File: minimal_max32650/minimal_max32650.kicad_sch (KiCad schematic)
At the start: 38 parts, among them J1 FTSH-105-01-L-DV-K, U1 MAX32650GCE+, U2 ADP225ACPZ-R7

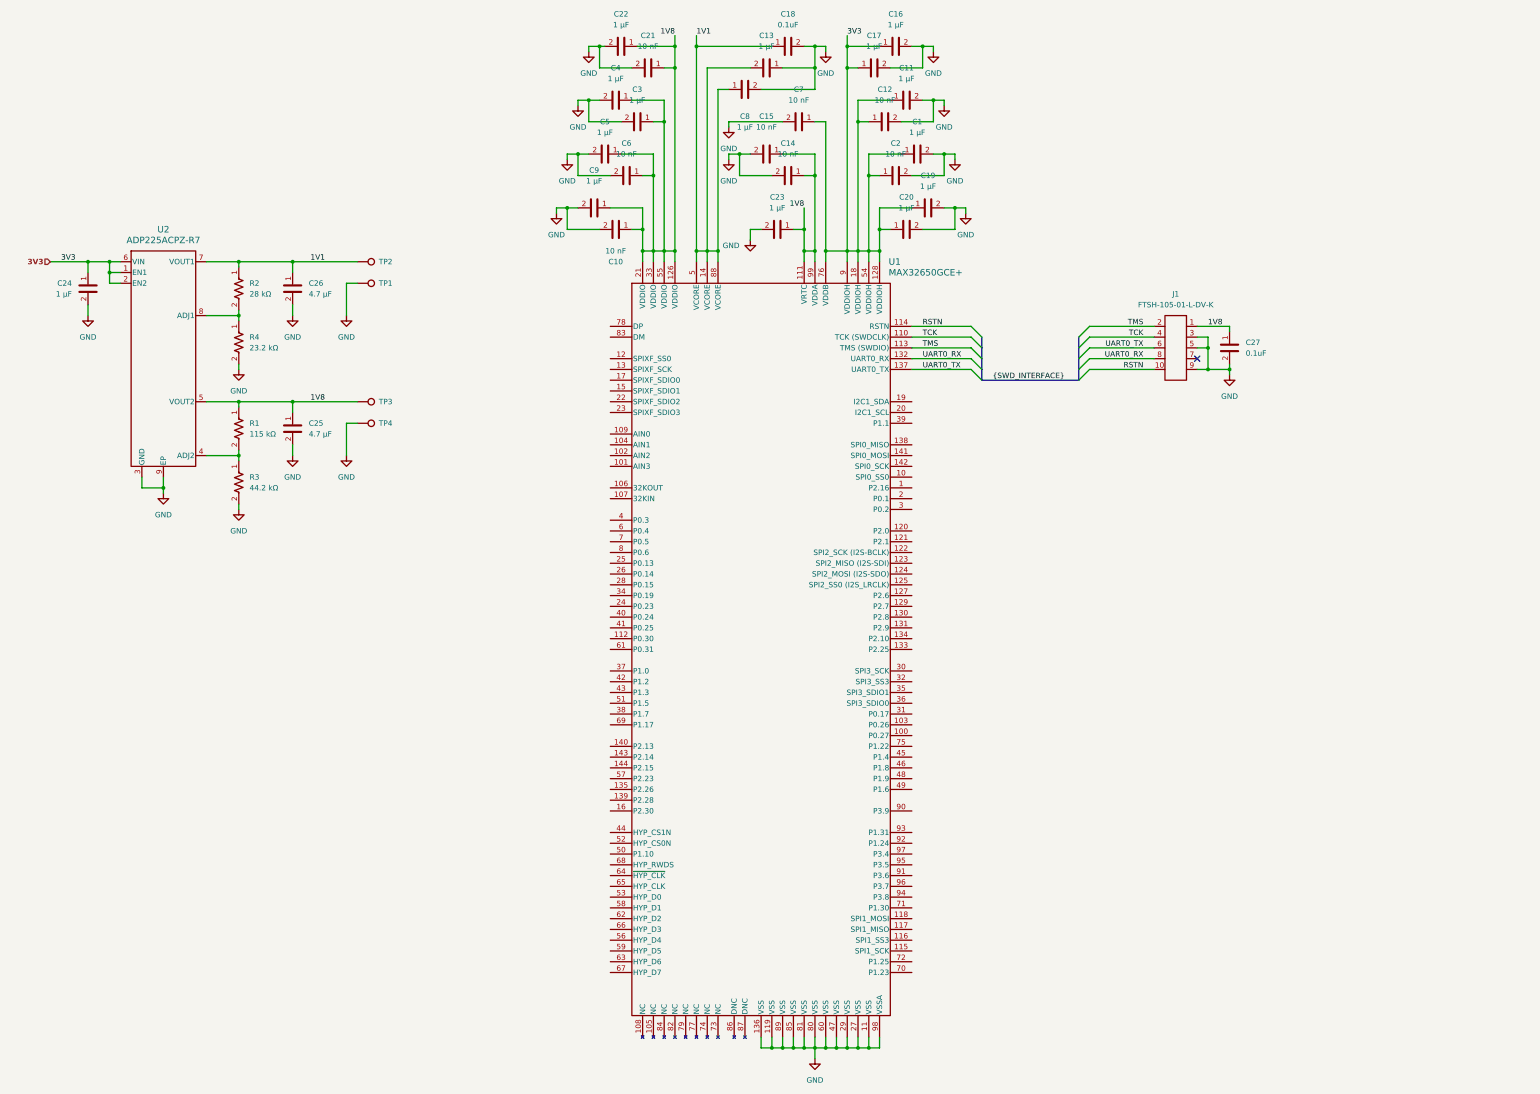
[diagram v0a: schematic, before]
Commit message: development backup
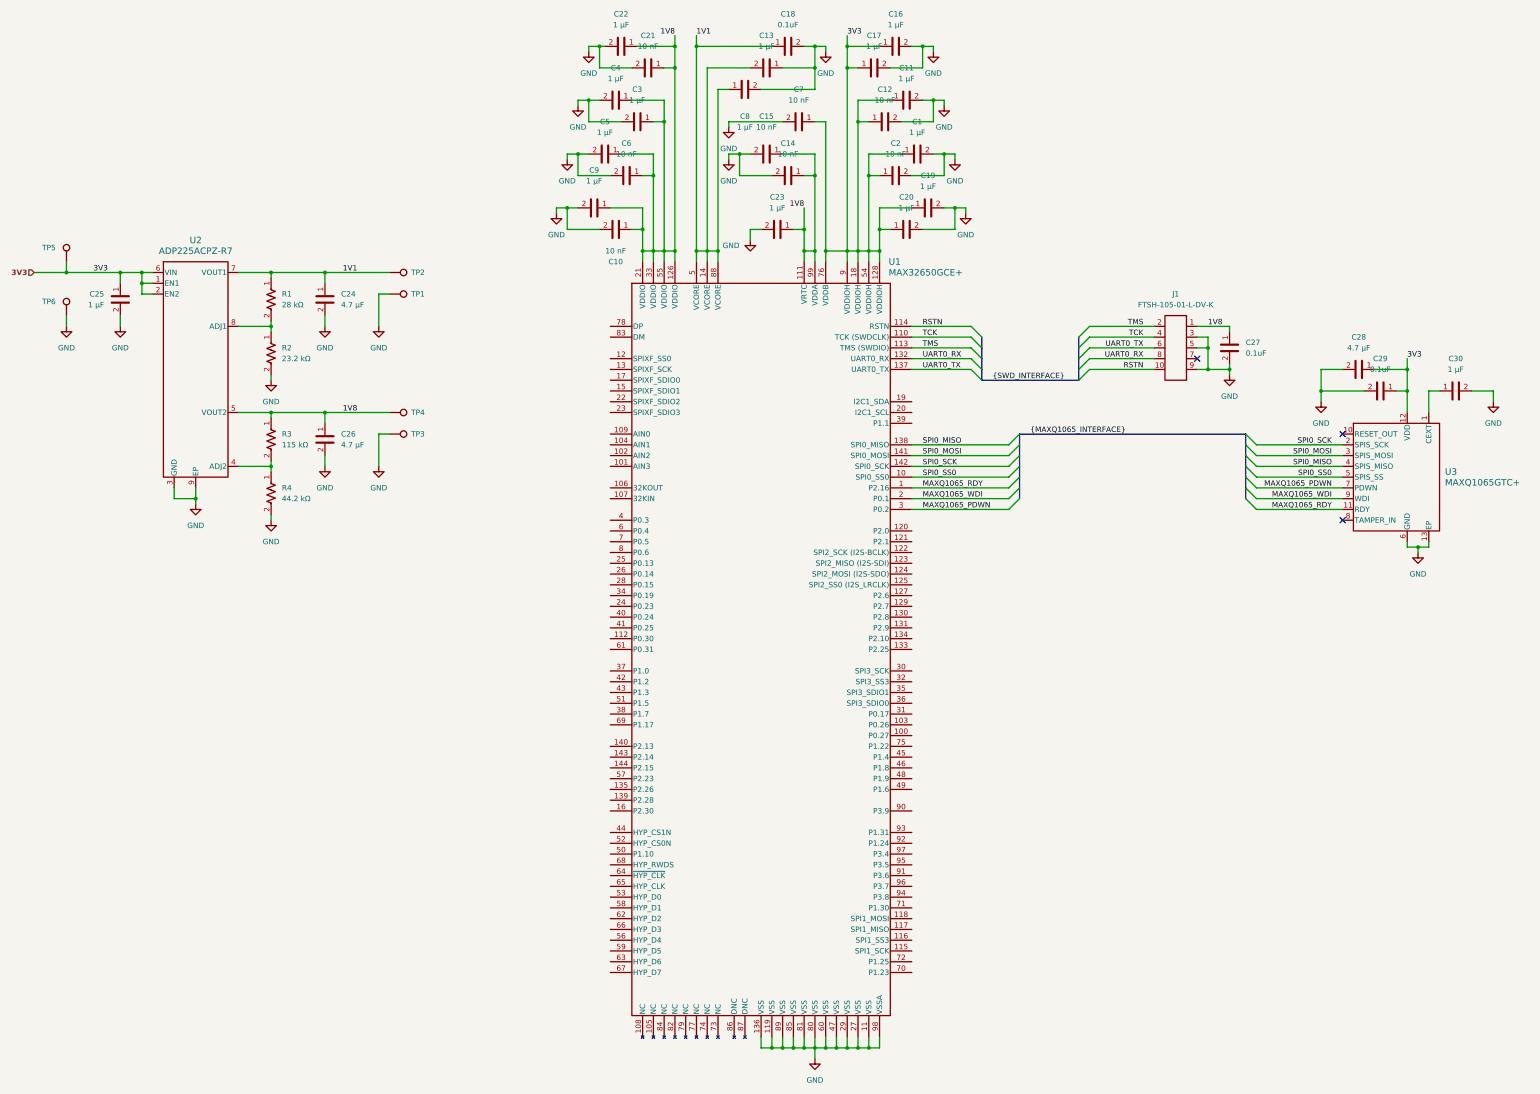
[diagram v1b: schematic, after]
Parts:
- added C28: 4.7 µF, capacitor_footprints:C_0603_1608Metric, symbol UNITED_CAPACITORS_DATA_BASE:C_C1608X7S1A475K080AC
- added C29: 0.1uF, capacitor_footprints:C_0402_1005Metric, symbol UNITED_CAPACITORS_DATA_BASE:C_GCM155R71H104KE02D
- added C30: 1 µF, capacitor_footprints:C_0402_1005Metric, symbol UNITED_CAPACITORS_DATA_BASE:C_C1005X6S1C105K050BC
- added TP5, TP6: TestPoint, test_point_footprints:TestPoint_THTPad_Castelated, symbol UNITED_TEST_POINTS:TestPoint_Castelated
- added U3: MAXQ1065GTC+, analog_devices_footprints:21-0664_TD1233&plus_1C_MXM, symbol UNITED_IC_ADI:U_MAXQ1065GTC+
- renumbered C26 to C24, C24 to C25, C25 to C26, R2 to R1, R4 to R2, R1 to R3, R3 to R4, TP4 to TP3, TP3 to TP4
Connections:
- net 3V3: now also C28.1, C29.1, TP5.1, U3.12 (VDD)
- net GND: now also C28.2, C29.2, C30.2, TP6.1, U3.13 (EP), U3.6 (GND)
- net MAXQ1065_RDY: now reaches U1.1 (P2.16)
- net MAXQ1065_RDY: now also U3.11 (RDY)
- net SPI0_SS0: now reaches U1.10 (P0.22)
- net SPI0_SS0: now also U3.5 (SPIS_SS)
- net SPI0_MISO: now reaches U1.138 (P3.1)
- net SPI0_MISO: now also U3.4 (SPIS_MISO)
- net SPI0_MOSI: now reaches U1.141 (P3.2)
- net SPI0_MOSI: now also U3.3 (SPIS_MOSI)
- net SPI0_SCK: now reaches U1.142 (P3.3)
- net SPI0_SCK: now also U3.2 (SPIS_SCK)
- net MAXQ1065_WDI: now reaches U1.2 (P0.1)
- net MAXQ1065_WDI: now also U3.9 (WDI)
- net MAXQ1065_PDWN: now reaches U1.3 (P0.2)
- net MAXQ1065_PDWN: now also U3.7 (PDWN)
- new net: C30.1, U3.1 (CEXT)
- no-connect marks 1 -> 3
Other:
- moved on the sheet: C24, C25, C26, C9, R1, R2, R3, R4, TP1, TP2, TP3, TP4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
